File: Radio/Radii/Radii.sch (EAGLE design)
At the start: 39 parts, among them J1 10118193-0001LF, J2 BUTTON, J3 BUTTON, J4 BUTTON, U2 ATMEGA32U4-AUR, U3 AP63203WU-7, U4 IND_1255AY-3R9N=P3, U8 BUTTON, U9 BUTTON, Y1 ECS-80-20-5PX-TR

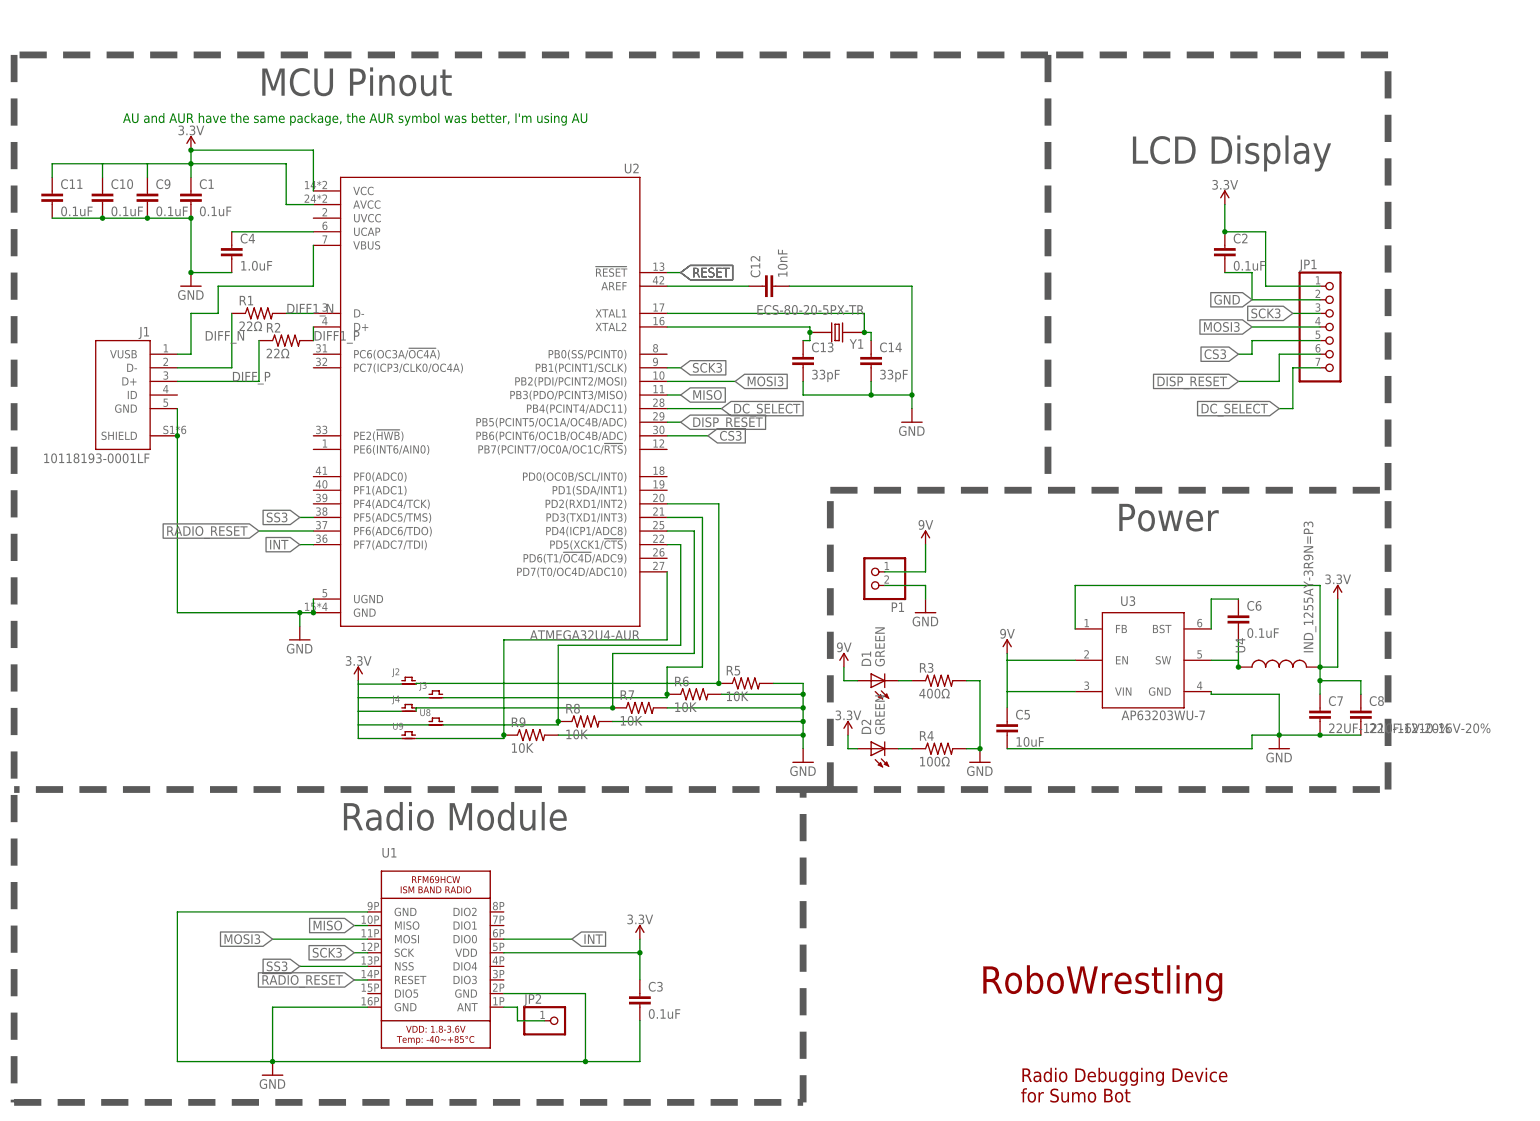
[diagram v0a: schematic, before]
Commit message: Added reset button
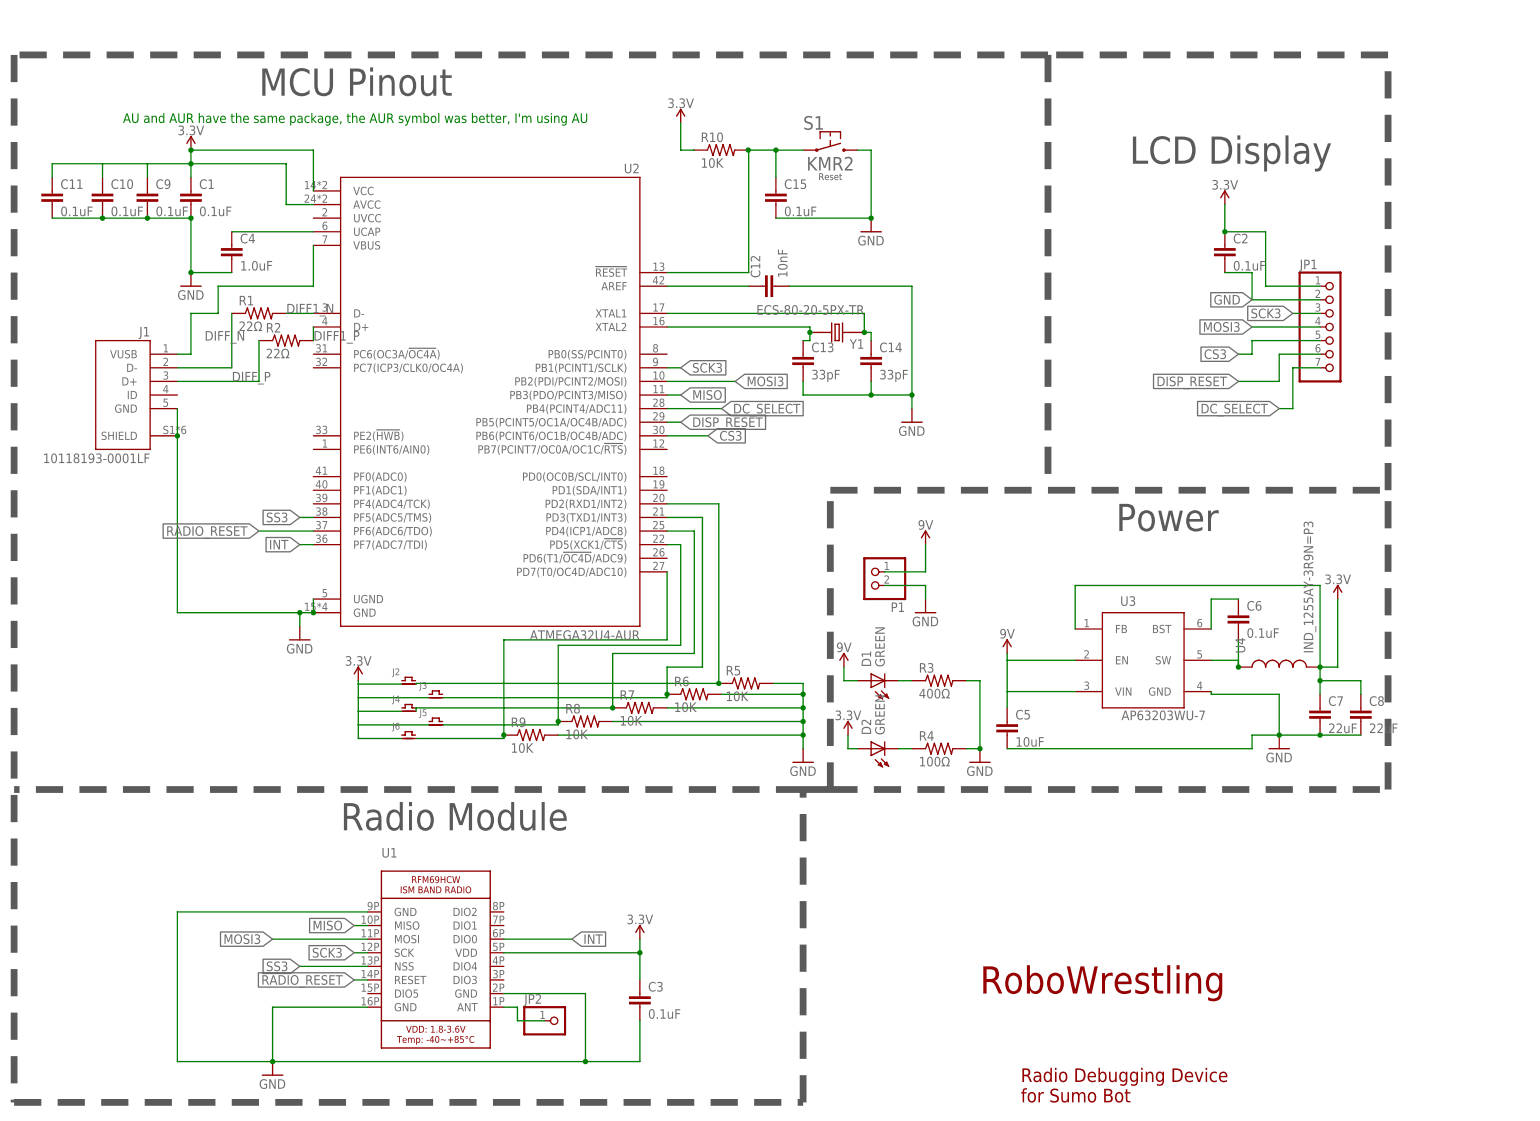
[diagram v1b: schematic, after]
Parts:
- added C15: 0.1uF, SparkFun-Capacitors:0.1UF-0603-25V-(+80/-20%)
- added R10: 10K, SparkFun-Resistors:10KOHM-1/10W-1%(0603)0603
- added S1: KMR2, RoboJackets-Switches:KMR2
- C7, C8: value 22UF-1210-16V-20% -> 22uF
- renumbered U8 to J5, U9 to J6
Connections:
- removed net RESET: U2.!RESET
- new net N$17: C15.1, R10.2, S1.1, U2.!RESET
- net 3.3V: now also R10.1
- net GND: now also C15.2, S1.2
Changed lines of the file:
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@@
 <part name="GND4" library="supply1" library_urn="urn:adsk.eagle:library:371" deviceset="GND" device=""/>
 <part name="SUPPLY7" library="SparkFun-PowerSymbols" library_urn="urn:adsk.eagle:library:530" deviceset="3.3V" device=""/>
-<part name="C7" library="SparkFun-Capacitors" library_urn="urn:adsk.eagle:library:510" deviceset="22UF" device="-1210-16V-20%" package3d_urn="urn:adsk.eagle:package:37436/1"/>
-<part name="C8" library="SparkFun-Capacitors" library_urn="urn:adsk.eagle:library:510" deviceset="22UF" device="-1210-16V-20%" package3d_urn="urn:adsk.eagle:package:37436/1"/>
+<part name="C7" library="SparkFun-Capacitors" library_urn="urn:adsk.eagle:library:510" deviceset="22UF" device="-1210-16V-20%" package3d_urn="urn:adsk.eagle:package:37436/1" value="22uF"/>
+<part name="C8" library="SparkFun-Capacitors" library_urn="urn:adsk.eagle:library:510" deviceset="22UF" device="-1210-16V-20%" package3d_urn="urn:adsk.eagle:package:37436/1" value="22uF"/>
 <part name="U4" library="I'mRADIOactive" deviceset="IND_1255AY-3R9N=P3" device=""/>
 <part name="SUPPLY5" library="SparkFun-PowerSymbols" library_urn="urn:adsk.eagle:library:530" deviceset="VCC_2" device="" value="9V"/>
@@
 <part name="J3" library="I'mRADIOactive" deviceset="BUTTON" device=""/>
 <part name="J4" library="I'mRADIOactive" deviceset="BUTTON" device=""/>
-<part name="U8" library="I'mRADIOactive" deviceset="BUTTON" device=""/>
-<part name="U9" library="I'mRADIOactive" deviceset="BUTTON" device=""/>
+<part name="J5" library="I'mRADIOactive" deviceset="BUTTON" device=""/>
+<part name="J6" library="I'mRADIOactive" deviceset="BUTTON" device=""/>
 <part name="SUPPLY9" library="SparkFun-PowerSymbols" library_urn="urn:adsk.eagle:library:530" deviceset="3.3V" device=""/>
 <part name="R5" library="SparkFun-Resistors" deviceset="10KOHM-1/10W-1%(0603)" device="0603" value="10K"/>
@@
 <part name="GND8" library="supply1" library_urn="urn:adsk.eagle:library:371" deviceset="GND" device=""/>
 <part name="R3" library="SparkFun-Resistors" deviceset="RESISTOR" device="0603" value="400Ω"/>
+<part name="S1" library="RoboJackets-Switches" deviceset="KMR2" device=""/>
+<part name="C15" library="SparkFun-Capacitors" library_urn="urn:adsk.eagle:library:510" deviceset="0.1UF" device="-0603-25V-(+80/-20%)" package3d_urn="urn:adsk.eagle:package:37414/1" value="0.1uF"/>
+<part name="SUPPLY10" library="SparkFun-PowerSymbols" library_urn="urn:adsk.eagle:library:530" deviceset="3.3V" device=""/>
+<part name="GND9" library="supply1" library_urn="urn:adsk.eagle:library:371" deviceset="GND" device=""/>
+<part name="R10" library="SparkFun-Resistors" deviceset="10KOHM-1/10W-1%(0603)" device="0603" value="10K"/>
 </parts>
 <sheets>
@@
 <attribute name="NAME" x="83.312" y="82.296" size="1.27" layer="95"/>
 </instance>
-<instance part="U8" gate="G$1" x="91.44" y="78.74" smashed="yes">
+<instance part="J5" gate="G$1" x="91.44" y="78.74" smashed="yes">
 <attribute name="NAME" x="88.392" y="79.756" size="1.27" layer="95"/>
 </instance>
-<instance part="U9" gate="G$1" x="86.36" y="76.2" smashed="yes">
+<instance part="J6" gate="G$1" x="86.36" y="76.2" smashed="yes">
 <attribute name="NAME" x="83.312" y="77.216" size="1.27" layer="95"/>
 </instance>
@@
 <attribute name="NAME" x="181.61" y="87.8586" size="1.778" layer="95"/>
 <attribute name="VALUE" x="181.61" y="83.058" size="1.778" layer="96"/>
+</instance>
+<instance part="S1" gate="G$1" x="165.1" y="185.42" smashed="yes">
+<attribute name="NAME" x="160.02" y="189.23" size="2.54" layer="95" font="vector"/>
+<attribute name="VALUE" x="165.1" y="184.15" size="2.54" layer="96" font="vector" ratio="15" align="top-center"/>
+<attribute name="FUNCTION" x="165.1" y="181.102" size="1.27" layer="97" ratio="10" align="top-center"/>
+</instance>
+<instance part="C15" gate="G$1" x="154.94" y="175.26" smashed="yes">
+<attribute name="NAME" x="156.464" y="178.181" size="1.778" layer="95" font="vector"/>
+<attribute name="VALUE" x="156.464" y="173.101" size="1.778" layer="96" font="vector"/>
+</instance>
+<instance part="SUPPLY10" gate="G$1" x="137.16" y="190.5" smashed="yes">
+<attribute name="VALUE" x="137.16" y="193.294" size="1.778" layer="96" align="bottom-center"/>
+</instance>
+<instance part="GND9" gate="1" x="172.72" y="170.18" smashed="yes">
+<attribute name="VALUE" x="170.18" y="167.64" size="1.778" layer="96"/>
+</instance>
+<instance part="R10" gate="G$1" x="144.697834375" y="185.43219375" smashed="yes">
+<attribute name="NAME" x="140.887834375" y="186.93079375" size="1.778" layer="95"/>
+<attribute name="VALUE" x="140.887834375" y="182.13019375" size="1.778" layer="96"/>
 </instance>
 </instances>
@@
 <wire x1="144.78" y1="83.82" x2="160.02" y2="83.82" width="0.1524" layer="91"/>
 <junction x="160.02" y="83.82"/>
+</segment>
+<segment>
+<pinref part="C15" gate="G$1" pin="2"/>
+<pinref part="GND9" gate="1" pin="GND"/>
+<wire x1="154.94" y1="172.72" x2="172.72" y2="172.72" width="0.1524" layer="91"/>
+<pinref part="S1" gate="G$1" pin="2"/>
+<wire x1="170.18" y1="185.42" x2="172.72" y2="185.42" width="0.1524" layer="91"/>
+<wire x1="172.72" y1="185.42" x2="172.72" y2="172.72" width="0.1524" layer="91"/>
+<junction x="172.72" y="172.72"/>
 </segment>
 </net>
@@
 <segment>
 <pinref part="SUPPLY9" gate="G$1" pin="3.3V"/>
-<pinref part="U9" gate="G$1" pin="P$1"/>
+<pinref part="J6" gate="G$1" pin="P$1"/>
 <wire x1="76.962" y1="86.36" x2="76.962" y2="85.725" width="0.1524" layer="91"/>
 <wire x1="76.962" y1="85.725" x2="76.962" y2="83.185" width="0.1524" layer="91"/>
@@
 <pinref part="J2" gate="G$1" pin="P$1"/>
 <wire x1="84.963" y1="85.725" x2="76.962" y2="85.725" width="0.1524" layer="91"/>
-<pinref part="U8" gate="G$1" pin="P$1"/>
+<pinref part="J5" gate="G$1" pin="P$1"/>
 <wire x1="90.043" y1="78.105" x2="76.962" y2="78.105" width="0.1524" layer="91"/>
+</segment>
+<segment>
+<pinref part="SUPPLY10" gate="G$1" pin="3.3V"/>
+<wire x1="137.16" y1="190.5" x2="137.16" y2="185.42" width="0.1524" layer="91"/>
+<pinref part="R10" gate="G$1" pin="1"/>
+<wire x1="137.16" y1="185.42" x2="139.617834375" y2="185.42" width="0.1524" layer="91"/>
+<wire x1="139.617834375" y1="185.42" x2="139.617834375" y2="185.43219375" width="0.1524" layer="91"/>
 </segment>
 </net>
@@
 <wire x1="134.62" y1="132.08" x2="142.24" y2="132.08" width="0.1524" layer="91"/>
 <label x="142.24" y="132.08" size="1.778" layer="95" xref="yes"/>
-</segment>
-</net>
-<net name="RESET" class="0">
-<segment>
-<label x="137.16" y="162.56" size="1.778" layer="95" xref="yes"/>
-<label x="137.16" y="162.56" size="1.778" layer="95" xref="yes"/>
-<label x="137.16" y="162.56" size="1.778" layer="95" xref="yes"/>
-<pinref part="U2" gate="G$1" pin="!RESET"/>
-<wire x1="137.16" y1="162.56" x2="134.62" y2="162.56" width="0.1524" layer="91"/>
 </segment>
 </net>
@@
 <net name="N$14" class="0">
 <segment>
-<pinref part="U8" gate="G$1" pin="P$2"/>
+<pinref part="J5" gate="G$1" pin="P$2"/>
 <pinref part="R8" gate="G$1" pin="1"/>
 <wire x1="92.837" y1="78.105" x2="114.3" y2="78.105" width="0.1524" layer="91"/>
@@
 <net name="N$15" class="0">
 <segment>
-<pinref part="U9" gate="G$1" pin="P$2"/>
+<pinref part="J6" gate="G$1" pin="P$2"/>
 <pinref part="R9" gate="G$1" pin="1"/>
 <wire x1="87.757" y1="75.565" x2="104.14" y2="75.565" width="0.1524" layer="91"/>
@@
 </segment>
 </net>
+<net name="N$17" class="0">
+<segment>
+<pinref part="S1" gate="G$1" pin="1"/>
+<wire x1="154.94" y1="185.42" x2="160.02" y2="185.42" width="0.1524" layer="91"/>
+<pinref part="C15" gate="G$1" pin="1"/>
+<wire x1="154.94" y1="180.34" x2="154.94" y2="185.42" width="0.1524" layer="91"/>
+<pinref part="R10" gate="G$1" pin="2"/>
+<wire x1="149.777834375" y1="185.43219375" x2="154.94" y2="185.43219375" width="0.1524" layer="91"/>
+<wire x1="154.94" y1="185.43219375" x2="154.94" y2="185.42" width="0.1524" layer="91"/>
+<junction x="154.94" y="185.42"/>
+<pinref part="U2" gate="G$1" pin="!RESET"/>
+<wire x1="134.62" y1="162.56" x2="149.86" y2="162.56" width="0.1524" layer="91"/>
+<wire x1="149.777834375" y1="185.43219375" x2="149.86" y2="185.43219375" width="0.1524" layer="91"/>
+<wire x1="149.86" y1="185.43219375" x2="149.86" y2="162.56" width="0.1524" layer="91"/>
+<junction x="149.777834375" y="185.43219375"/>
+</segment>
+</net>

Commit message: Fixed a couple parts of Radii PCB
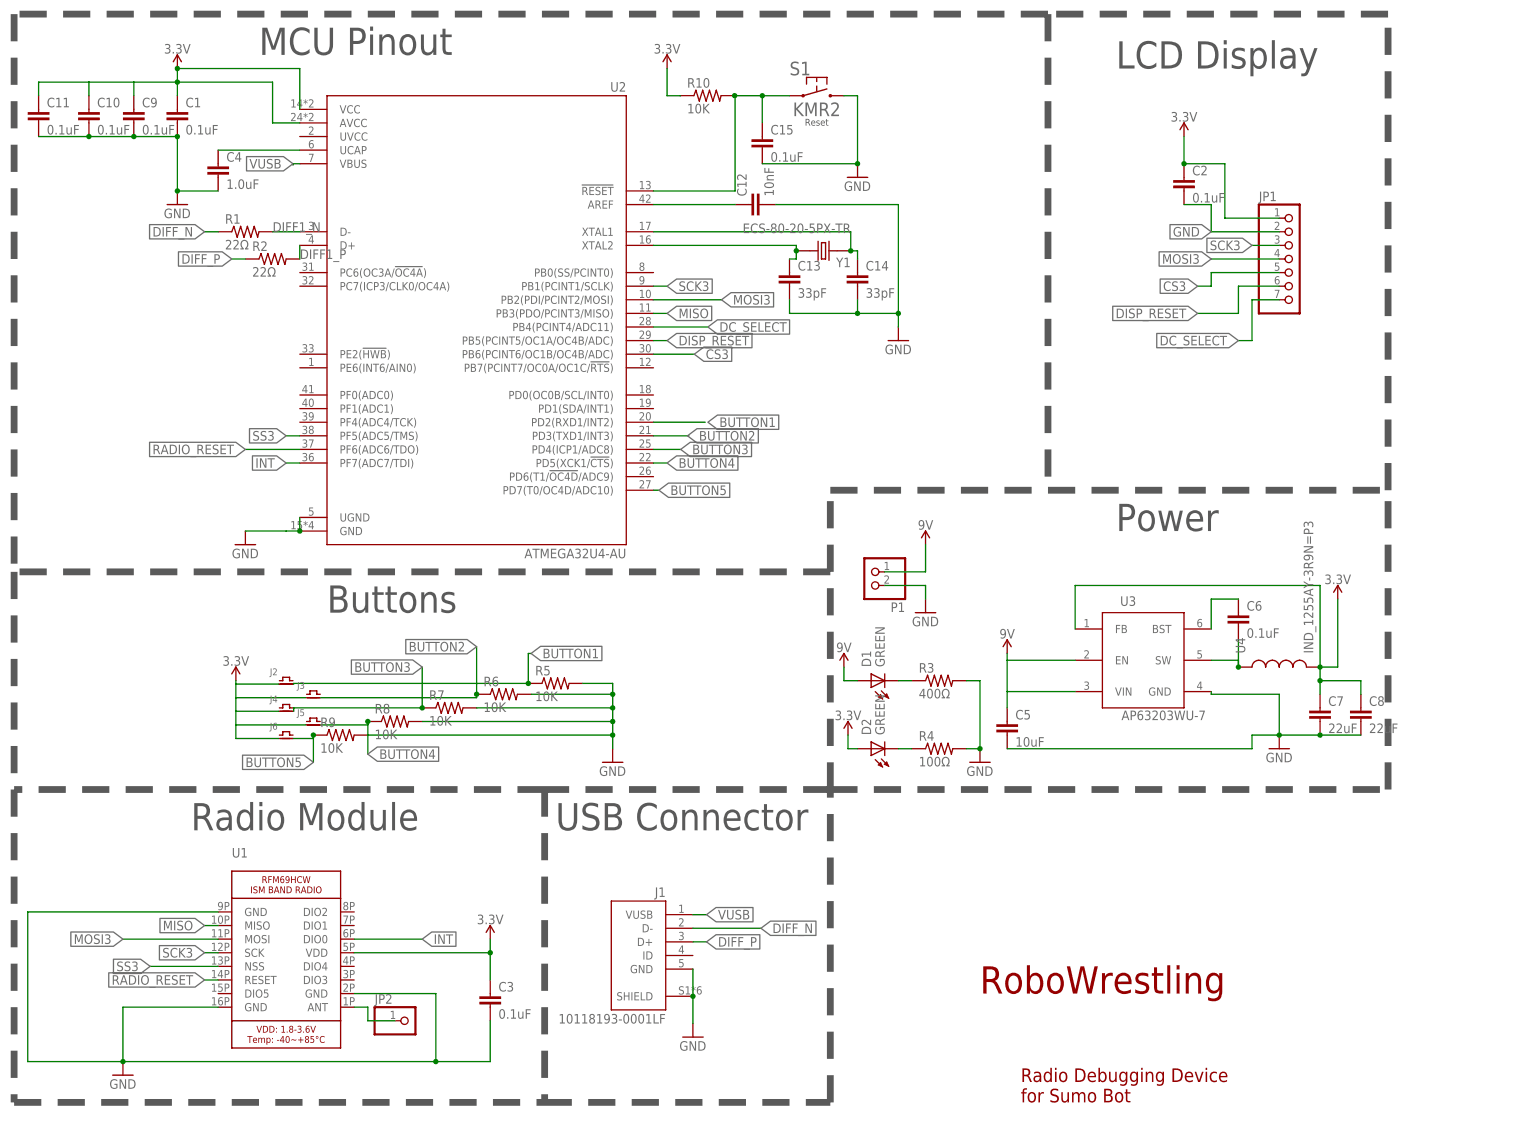
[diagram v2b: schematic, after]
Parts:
- U2: value ATMEGA32U4-AUR -> ATMEGA32U4-AU
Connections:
- net N$11 renamed BUTTON1
- net N$12 renamed BUTTON2
- net N$13 renamed BUTTON3
- net N$14 renamed BUTTON4
- net N$15 renamed BUTTON5
- net N$4 renamed VUSB
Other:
- note added: "Buttons"
- note added: "USB Connector"
- note removed: "AU and AUR have the same package, the AUR symbol was better, I'm using AU"
- moved on the sheet: C1, C10, C11, C12, C13, C14, C15, C2, C3, C4, C9, J1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
